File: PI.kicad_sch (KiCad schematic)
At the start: 45 parts, among them Q3 2SC1815, Q4 MTBT3906, Q5 MTBT3904, Q6 2SD1415A, Q7 TTB1020B, Q8 2SD1415A, Q9 TTB1020B, U12 KIA75S358F, U4 ADA4522-1ARZ

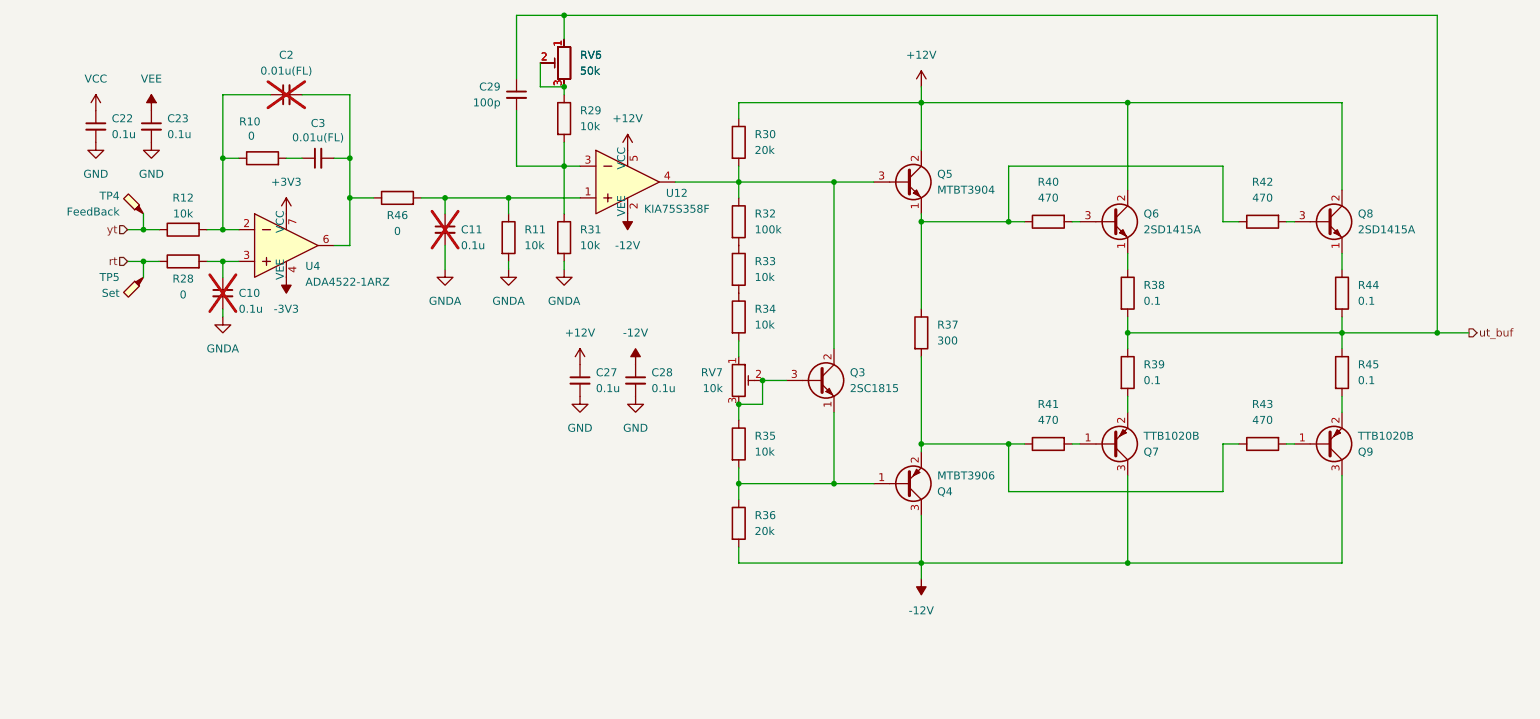
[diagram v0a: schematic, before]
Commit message: aaaa
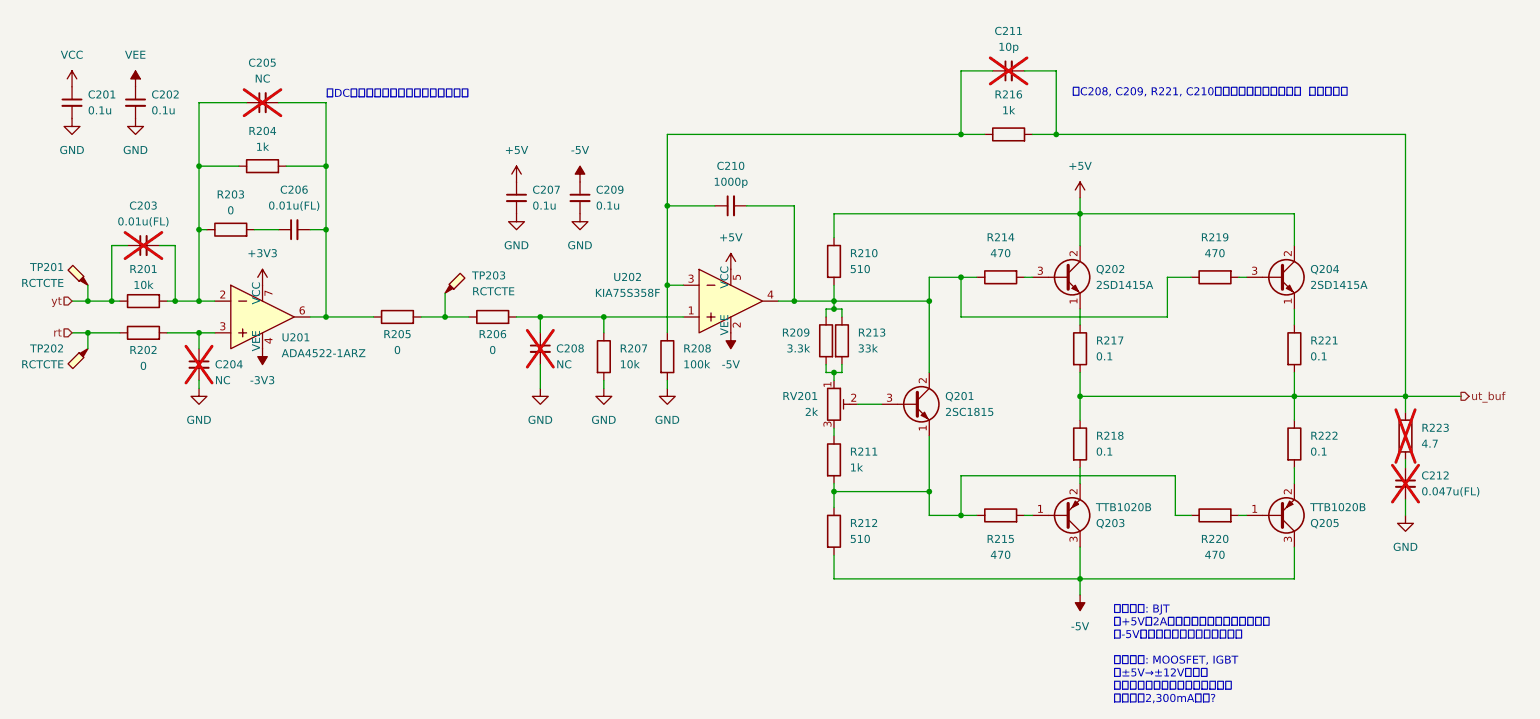
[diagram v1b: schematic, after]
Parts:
- removed C2: 0.01u(FL), Capacitor_THT:C_Rect_L7.0mm_W2.5mm_P5.00mm, symbol Device:C_Small
- removed C29: 100p, Capacitor_SMD:C_0603_1608Metric, symbol Device:C_Small
- removed Q4: MTBT3906, Package_TO_SOT_THT:TO-92S, symbol Transistor_BJT:Q_PNP_BEC
- removed Q5: MTBT3904, symbol Transistor_BJT:Q_NPN_ECB
- removed R10: 0, Resistor_THT:R_Axial_DIN0207_L6.3mm_D2.5mm_P2.54mm_Vertical, symbol Device:R
- removed R29, R33: 10k, symbol Device:R
- removed R32: 100k, symbol Device:R
- removed R37: 300, symbol Device:R
- removed RV5, RV6: 50k, symbol Device:R_Potentiometer_Trim
- added C203: 0.01u(FL), Capacitor_SMD:C_0805_2012Metric, symbol Device:C_Small
- added C205: NC, Capacitor_SMD:C_0805_2012Metric, symbol Device:C_Small
- added C210: 1000p, Capacitor_SMD:C_0805_2012Metric, symbol Device:C_Small
- added C211: 10p, Capacitor_SMD:C_0603_1608Metric, symbol Device:C_Small
- added C212: 0.047u(FL), Capacitor_THT:C_Rect_L7.2mm_W5.0mm_P5.00mm, symbol Device:C_Small
- added R203, R205: 0, Resistor_SMD:R_0603_1608Metric, symbol Device:R
- added R204, R216: 1k, Resistor_SMD:R_0603_1608Metric, symbol Device:R
- added R213: 33k, Resistor_SMD:R_0603_1608Metric, symbol Device:R
- added R223: 4.7, Resistor_SMD:R_2512_6332Metric, symbol Device:R
- added TP203: RCTCTE, symbol Connector:TestPoint_Probe
- C201: renamed from C22; Akizuki_code (none) -> 105728
- C202: renamed from C23; Akizuki_code (none) -> 105728
- C204: renamed from C10; value 0.1u -> NC
- C206: renamed from C3; footprint Capacitor_THT:C_Rect_L7.0mm_W2.5mm_P5.00mm -> Capacitor_SMD:C_0805_2012Metric; Akizuki_code 116112 -> 115631
- C207: renamed from C27; Akizuki_code (none) -> 105728
- C208: renamed from C11; value 0.1u -> NC
- C209: renamed from C28; Akizuki_code (none) -> 105728
- Q201: renamed from Q3; footprint (none) -> Package_TO_SOT_THT:TO-92L_Inline; Akizuki_code (none) -> 117089
- Q202: renamed from Q6; footprint (none) -> Package_TO_SOT_THT:TO-220-3_Vertical; Akizuki_code (none) -> 110058; Akizuki_code2 (none) -> 106369
- Q203: renamed from Q7; footprint Package_TO_SOT_THT:TO-92S -> Package_TO_SOT_THT:TO-220-3_Vertical; Akizuki_code (none) -> 117309
- Q204: renamed from Q8; footprint (none) -> Package_TO_SOT_THT:TO-220-3_Vertical; Akizuki_code (none) -> 110058; Akizuki_code2 (none) -> 106369
- Q205: renamed from Q9; footprint Package_TO_SOT_THT:TO-92S -> Package_TO_SOT_THT:TO-220-3_Vertical; Akizuki_code (none) -> 117309
- R201: renamed from R12; footprint Resistor_THT:R_Axial_DIN0207_L6.3mm_D2.5mm_P2.54mm_Vertical -> Resistor_SMD:R_0603_1608Metric; Akizuki_code (none) -> 106668
- R202: renamed from R28; footprint Resistor_THT:R_Axial_DIN0207_L6.3mm_D2.5mm_P2.54mm_Vertical -> Resistor_SMD:R_0603_1608Metric
- R206: renamed from R46; footprint Resistor_THT:R_Axial_DIN0207_L6.3mm_D2.5mm_P2.54mm_Vertical -> Resistor_SMD:R_0603_1608Metric
- R207: renamed from R11; footprint Resistor_THT:R_Bare_Metal_Element_L16.3mm_W4.8mm_P15.30mm -> Resistor_SMD:R_0603_1608Metric
- R208: renamed from R31; value 10k -> 100k; footprint Resistor_THT:R_Bare_Metal_Element_L16.3mm_W4.8mm_P15.30mm -> Resistor_SMD:R_0603_1608Metric
- R209: renamed from R34; value 10k -> 3.3k; footprint (none) -> Resistor_SMD:R_0603_1608Metric
- R210: renamed from R30; value 20k -> 510; footprint (none) -> Resistor_SMD:R_2512_6332Metric; Sengoku_code (none) -> EEHD-0ECM
- R211: renamed from R35; value 10k -> 1k; footprint (none) -> Resistor_SMD:R_0805_2012Metric; Sengoku_code (none) -> EEHD-57BZ
- R212: renamed from R36; value 20k -> 510; footprint (none) -> Resistor_SMD:R_2512_6332Metric; Sengoku_code (none) -> EEHD-0ECM
- R214: renamed from R40; footprint (none) -> Resistor_SMD:R_1206_3216Metric; Sengoku_code (none) -> EEHD-57BS
- R215: renamed from R41; footprint (none) -> Resistor_SMD:R_1206_3216Metric; Sengoku_code (none) -> EEHD-57BS
- R219: renamed from R42; footprint (none) -> Resistor_SMD:R_1206_3216Metric; Sengoku_code (none) -> EEHD-57BS
- R220: renamed from R43; footprint (none) -> Resistor_SMD:R_1206_3216Metric; Sengoku_code (none) -> EEHD-57BS
- RV201: renamed from RV7; value 10k -> 2k; footprint (none) -> AM_Potentiometer:TSR-065-xxx-R
- TP201: renamed from TP4; value FeedBack -> RCTCTE; footprint TestPoint:TestPoint_Loop_D2.50mm_Drill1.0mm -> (none)
- TP202: renamed from TP5; value Set -> RCTCTE; footprint TestPoint:TestPoint_Loop_D2.50mm_Drill1.0mm -> (none)
- U201: renamed from U4; footprint Package_DIP:DIP-8_W7.62mm -> Package_SO:SOIC-8_3.9x4.9mm_P1.27mm; AkizukiCode 114063 -> (none); Akizuki_code2 (none) -> 114063
- renumbered R38 to R217, R39 to R218, R44 to R221, R45 to R222, U12 to U202
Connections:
- net GNDA is gone; now on net GND: C204.2, C208.2, R207.2, R208.2
- net GND: now also C212.2
- net ut_buf: now also C211.2, R216.2, R223.1
- net yt: now also C203.1
- net at C206.2, U201.6: now also C205.2, R204.2, R205.1; no longer R206.1
- net at R214.1, R219.1: now also Q201.2 (C), R209.1, R210.2, U202.4, C210.2, R213.1
- net at R215.1, R220.1: now also Q201.1 (E), R211.2, R212.1
- net at R208.1, U202.3: now also C210.1, C211.1, R216.1
- net at R201.2, U201.2: now also C203.2, C205.1, R203.1, R204.1
- net at R209.2, RV201.1: now also R213.2
- net at C206.1: now also R203.2
- net at R211.1, RV201.3: no longer Q201.3 (B), RV201.2
- net +12V renamed +5V
- net -12V renamed -5V
- new net: R205.2, R206.1, TP203.1
- new net: C212.1, R223.2
- new net: Q201.3 (B), RV201.2
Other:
- note added: "・C208, C209, R221, C210は発振止めのオプション 適宜つける"
- note added: "・DCゲインあげすぎると多分発振する"
- note added: "負荷素子: BJT ・+5Vは2A位の容量はとれるようにする ・-5Vは動作しないので適当な容量 負荷素子: MOOSFET, IGBT ・±5V→±12Vに変更 ・適当にバイアスの抵抗も変える ・電源は2,300mA程度?"
- moved on the sheet: C201, C202, C204, C206, C207, C208, C209, Q201, Q202, Q203, Q204, Q205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
